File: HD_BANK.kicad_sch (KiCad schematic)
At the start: 1 part, among them J6 Conn_02x70_Odd_Even

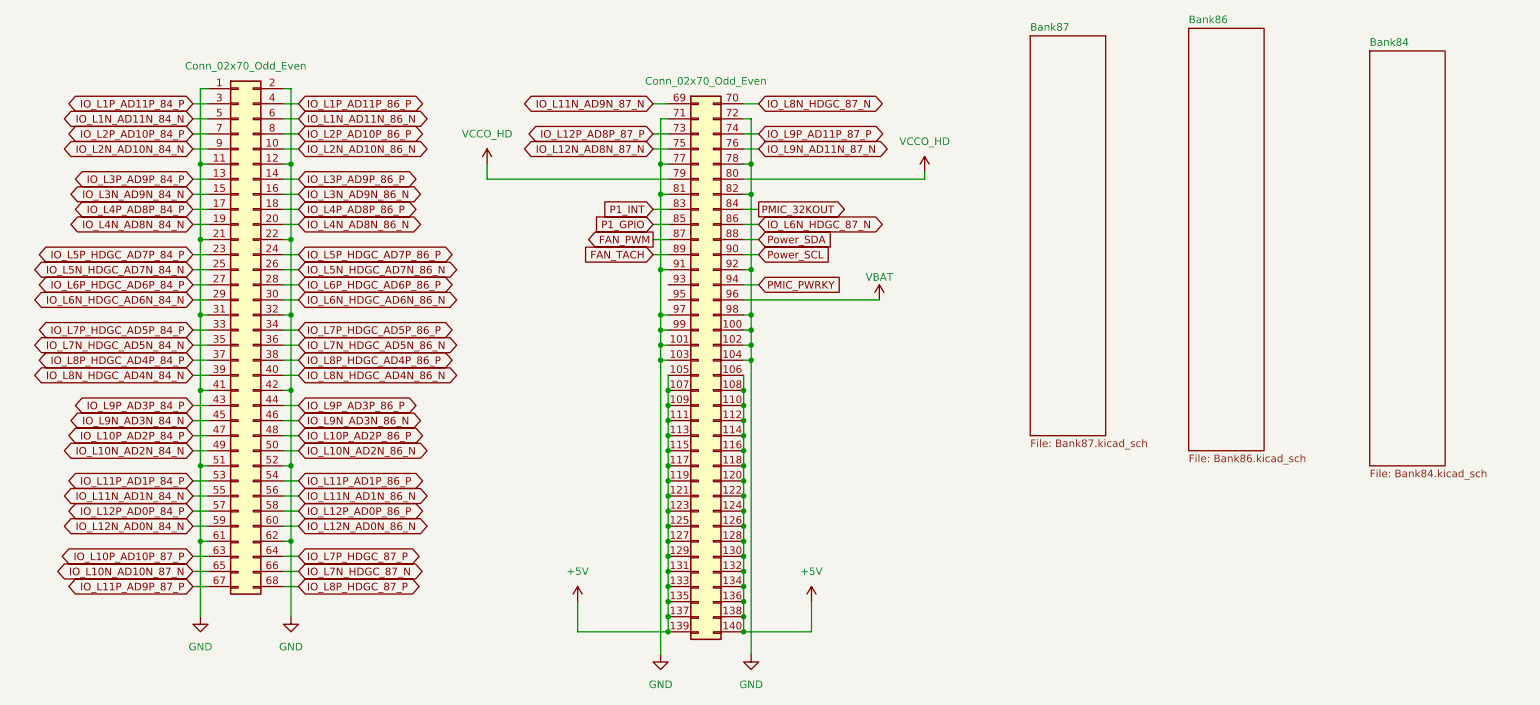
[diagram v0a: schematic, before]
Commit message: pushing the schematics works
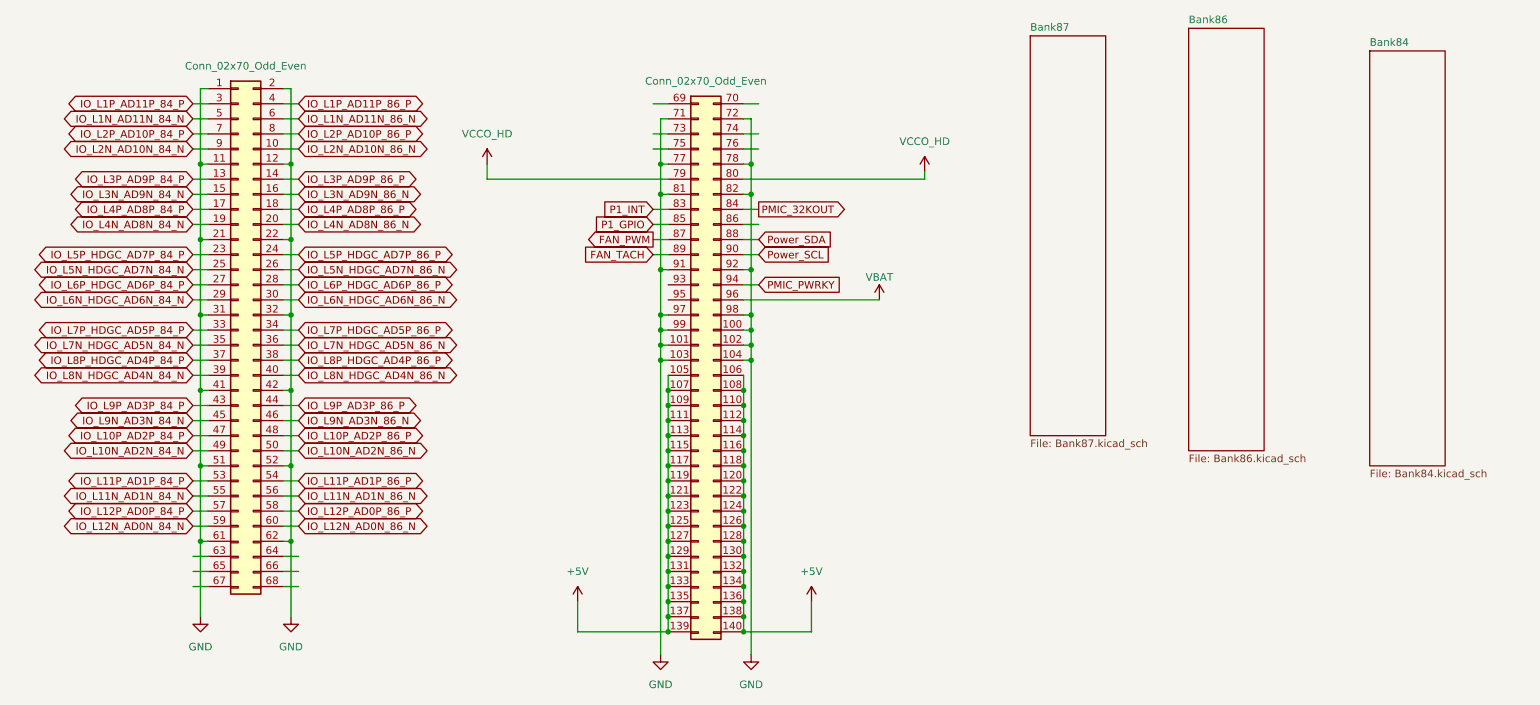
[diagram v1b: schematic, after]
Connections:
- net IO_L10N_AD10N_87_N: no longer names the net of J6.65 (Pin_65)
- net IO_L10P_AD10P_87_P: no longer names the net of J6.63 (Pin_63)
- net IO_L11N_AD9N_87_N: no longer names the net of J6.69 (Pin_69)
- net IO_L11P_AD9P_87_P: no longer names the net of J6.67 (Pin_67)
- net IO_L12N_AD8N_87_N: no longer names the net of J6.75 (Pin_75)
- net IO_L12P_AD8P_87_P: no longer names the net of J6.73 (Pin_73)
- net IO_L6N_HDGC_87_N: no longer names the net of J6.86 (Pin_86)
- net IO_L7N_HDGC_87_N: no longer names the net of J6.66 (Pin_66)
- net IO_L7P_HDGC_87_P: no longer names the net of J6.64 (Pin_64)
- net IO_L8N_HDGC_87_N: no longer names the net of J6.70 (Pin_70)
- net IO_L8P_HDGC_87_P: no longer names the net of J6.68 (Pin_68)
- net IO_L9N_AD11N_87_N: no longer names the net of J6.76 (Pin_76)
- net IO_L9P_AD11P_87_P: no longer names the net of J6.74 (Pin_74)
